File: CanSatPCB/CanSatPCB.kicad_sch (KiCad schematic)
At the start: 1 part, among them U1 ESP32-S3-MINI-1U

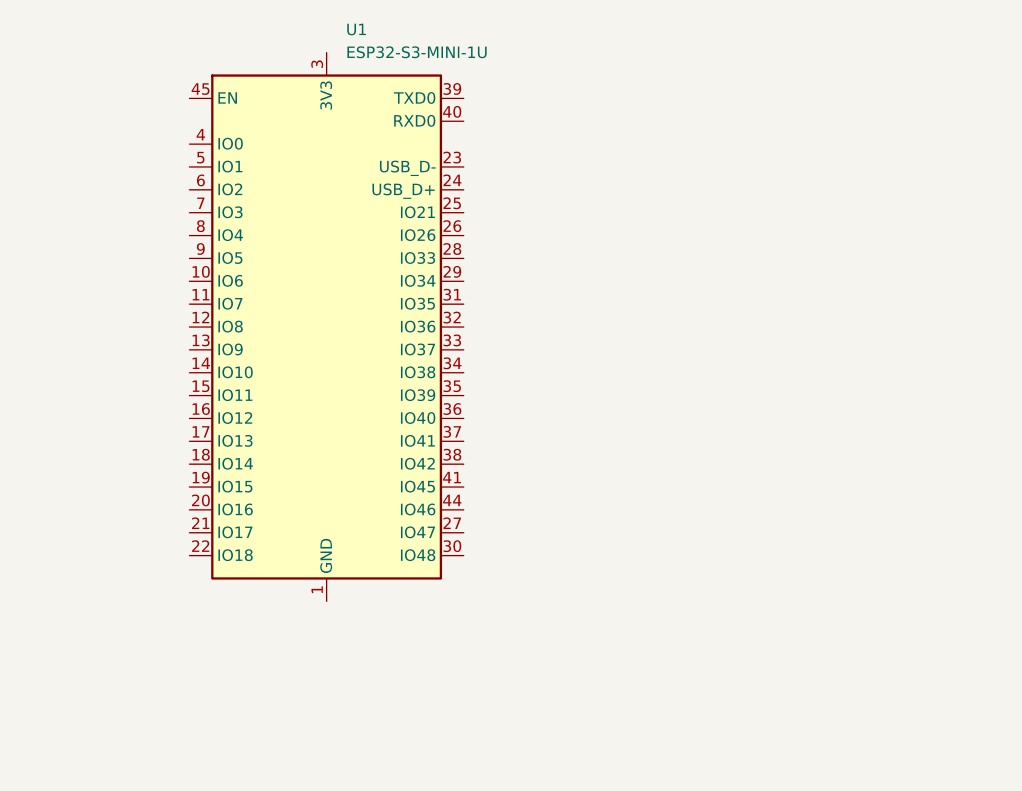
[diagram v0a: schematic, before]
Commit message: last test for the git ignore
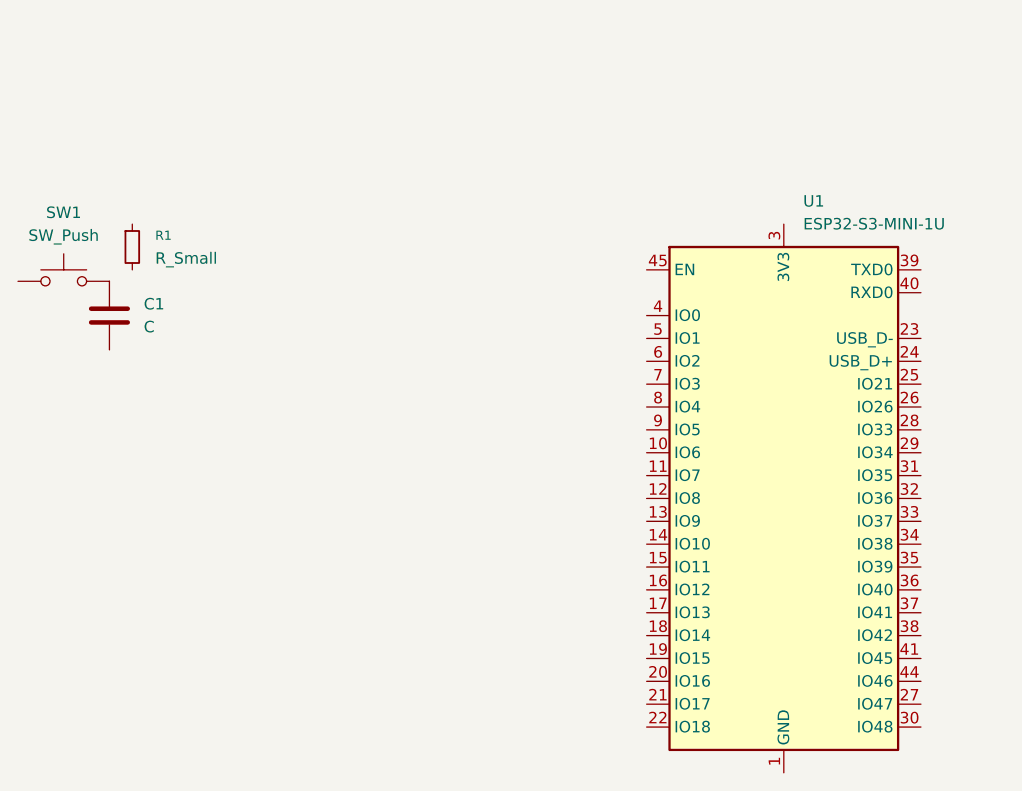
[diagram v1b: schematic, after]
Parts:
- added C1: C, symbol Device:C
- added R1: R_Small, symbol Device:R_Small
- added SW1: SW_Push, symbol Switch:SW_Push
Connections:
- new net: C1.1, SW1.2
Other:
- moved on the sheet: U1
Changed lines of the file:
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@@
 	(paper "A4")
 	(symbol
+		(lib_id "Device:R_Small")
+		(at 78.74 45.72 0)
+		(unit 1)
+		(exclude_from_sim no)
+		(in_bom yes)
+		(on_board yes)
+		(dnp no)
+		(fields_autoplaced yes)
+		(property "Reference" "R1"
+			(at 81.28 44.4499 0)
+			(effects
+				(font
+					(size 1.016 1.016)
+				)
+				(justify left)
+			)
+		)
+		(property "Value" "R_Small"
+			(at 81.28 46.9899 0)
+			(effects
+				(font
+					(size 1.27 1.27)
+				)
+				(justify left)
+			)
+		)
+		(property "Footprint" ""
+			(at 78.74 45.72 0)
+			(effects
+				(font
+					(size 1.27 1.27)
+				)
+				(hide yes)
+			)
+		)
+		(property "Datasheet" "~"
+			(at 78.74 45.72 0)
+			(effects
+				(font
+					(size 1.27 1.27)
+				)
+				(hide yes)
+			)
+		)
+		(property "Description" "Resistor, small symbol"
+			(at 78.74 45.72 0)
+			(effects
+				(font
+					(size 1.27 1.27)
+				)
+				(hide yes)
+			)
+		)
+		(pin "1"
+		)
+		(pin "2"
+		)
+		(instances
+			(project ""
+				(path "/a1548337-1355-40e9-bc99-5140aa8d75a0"
+					(reference "R1")
+					(unit 1)
+				)
+			)
+		)
+	)
+	(symbol
 		(lib_id "RF_Module:ESP32-S3-MINI-1U")
-		(at 100.33 54.61 0)
+		(at 151.13 73.66 0)
 		(unit 1)
 		(exclude_from_sim no)
@@
 		(fields_autoplaced yes)
 		(property "Reference" "U1"
-			(at 102.4733 21.59 0)
+			(at 153.2733 40.64 0)
 			(effects
 				(font
@@
 		)
 		(property "Value" "ESP32-S3-MINI-1U"
-			(at 102.4733 24.13 0)
+			(at 153.2733 43.18 0)
 			(effects
 				(font
@@
 		)
 		(property "Footprint" "RF_Module:ESP32-S2-MINI-1U"
-			(at 116.84 83.82 0)
+			(at 167.64 102.87 0)
 			(effects
 				(font
@@
 		)
 		(property "Datasheet" "https://www.espressif.com/sites/default/files/documentation/esp32-s3-mini-1_mini-1u_datasheet_en.pdf"
-			(at 100.33 13.97 0)
+			(at 151.13 33.02 0)
 			(effects
 				(font
@@
 		)
 		(property "Description" "RF Module, ESP32-S3 SoC, Wi-Fi 802.11b/g/n, Bluetooth, BLE, 32-bit, 3.3V, SMD, external antenna"
-			(at 100.33 11.43 0)
+			(at 151.13 30.48 0)
 			(effects
 				(font
@@
 					(unit 1)
 				)
+			)
+		)
+	)
+	(symbol
+		(lib_id "Device:C")
+		(at 76.2 53.34 0)
+		(unit 1)
+		(exclude_from_sim no)
+		(in_bom yes)
+		(on_board yes)
+		(dnp no)
+		(fields_autoplaced yes)
+		(property "Reference" "C1"
+			(at 80.01 52.0699 0)
+			(effects
+				(font
+					(size 1.27 1.27)
+				)
+				(justify left)
+			)
+		)
+		(property "Value" "C"
+			(at 80.01 54.6099 0)
+			(effects
+				(font
+					(size 1.27 1.27)
+				)
+				(justify left)
+			)
+		)
+		(property "Footprint" ""
+			(at 77.1652 57.15 0)
+			(effects
+				(font
+					(size 1.27 1.27)
+				)
+				(hide yes)
+			)
+		)
+		(property "Datasheet" "~"
+			(at 76.2 53.34 0)
+			(effects
+				(font
+					(size 1.27 1.27)
+				)
+				(hide yes)
+			)
+		)
+		(property "Description" "Unpolarized capacitor"
+			(at 76.2 53.34 0)
+			(effects
+				(font
+					(size 1.27 1.27)
+				)
+				(hide yes)
+			)
+		)
+		(pin "1"
+		)
+		(pin "2"
+		)
+		(instances
+			(project ""
+				(path "/a1548337-1355-40e9-bc99-5140aa8d75a0"
+					(reference "C1")
+					(unit 1)
+				)
+			)
+		)
+	)
+	(symbol
+		(lib_id "Switch:SW_Push")
+		(at 71.12 49.53 0)
+		(unit 1)
+		(exclude_from_sim no)
+		(in_bom yes)
+		(on_board yes)
+		(dnp no)
+		(fields_autoplaced yes)
+		(property "Reference" "SW1"
+			(at 71.12 41.91 0)
+			(effects
+				(font
+					(size 1.27 1.27)
+				)
+			)
+		)
+		(property "Value" "SW_Push"
+			(at 71.12 44.45 0)
+			(effects
+				(font
+					(size 1.27 1.27)
+				)
+			)
+		)
+		(property "Footprint" ""
+			(at 71.12 44.45 0)
+			(effects
+				(font
+					(size 1.27 1.27)
+				)
+				(hide yes)
+			)
+		)
+		(property "Datasheet" "~"
+			(at 71.12 44.45 0)
+			(effects
+				(font
+					(size 1.27 1.27)
+				)
+				(hide yes)
+			)
+		)
+		(property "Description" "Push button switch, generic, two pins"
+			(at 71.12 49.53 0)
+			(effects
+				(font
+					(size 1.27 1.27)
+				)
+				(hide yes)
+			)
+		)
+		(pin "1"
+		)
+		(pin "2"
+		)
+		(instances
+			(project ""
+				(path "/a1548337-1355-40e9-bc99-5140aa8d75a0"
+					(reference "SW1")
+					(unit 1)
+				)
